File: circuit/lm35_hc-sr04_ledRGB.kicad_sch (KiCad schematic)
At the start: 4 parts, among them U1 LM35-D, U3 HC-SR04

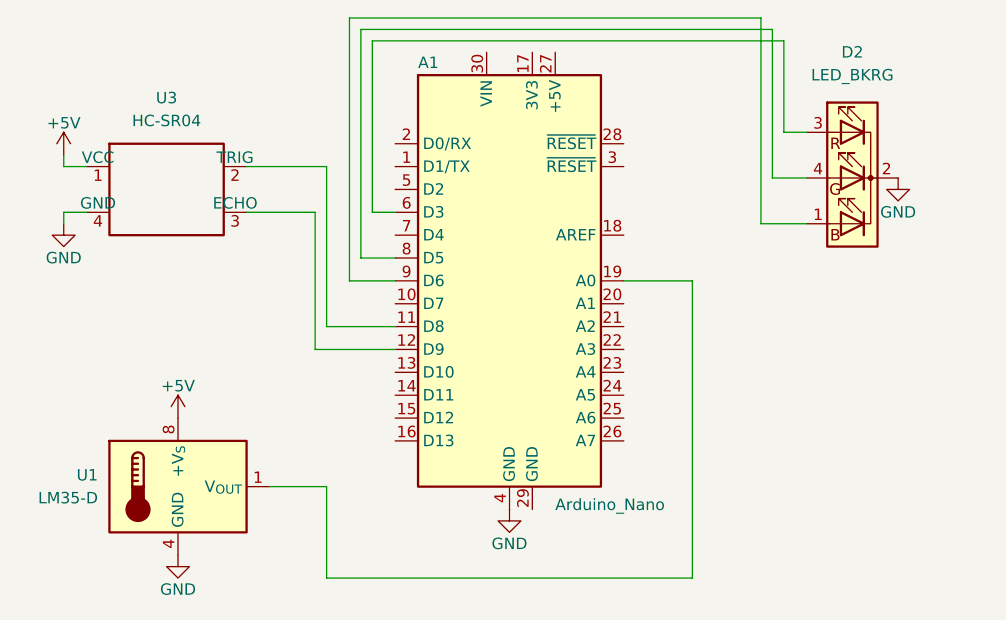
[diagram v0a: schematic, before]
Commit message: guarde circuito
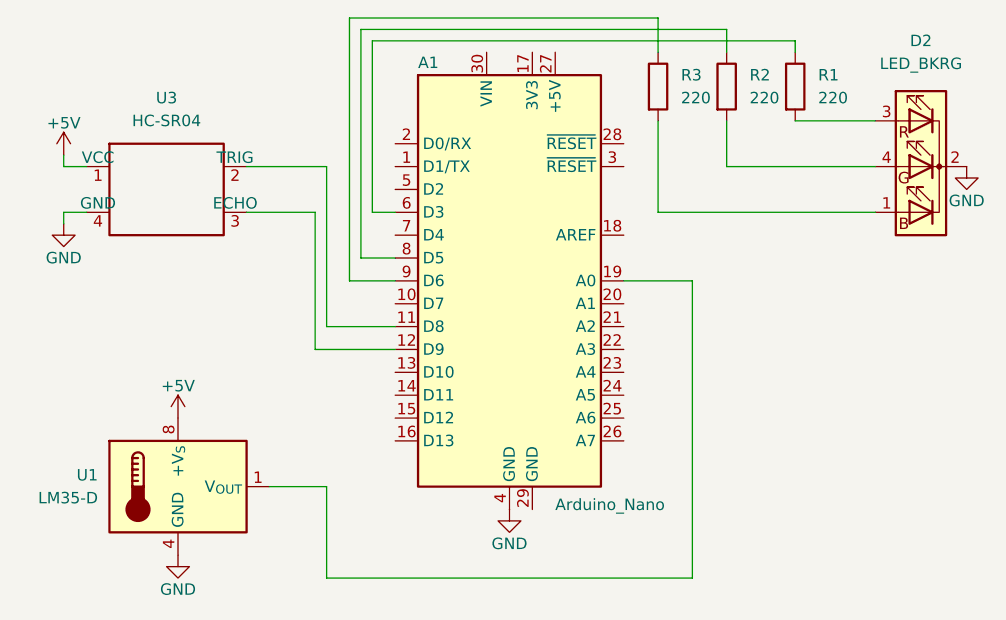
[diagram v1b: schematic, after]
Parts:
- added R1, R2, R3: 220, symbol Device:R
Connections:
- net at D2.1 (BA): now also R3.2; no longer A1.9 (D6)
- net at D2.3 (RA): now also R1.2; no longer A1.6 (D3)
- net at A1.8 (D5): now also R2.1; no longer D2.4 (GA)
- new net: D2.4 (GA), R2.2
- new net: A1.6 (D3), R1.1
- new net: A1.9 (D6), R3.1
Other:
- moved on the sheet: D2
